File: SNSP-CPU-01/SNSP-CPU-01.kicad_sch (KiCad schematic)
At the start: 400 parts, among them J1 Jack-DC, J3 Conn_02x06_Odd_Even, J4 CONTROLLER 1, J5 CONTROLLER 2, P1 CASSETTE, P2 JST 11FE-BT-VK-N, P3 Conn_01x02_Pin, P7 JST 11FE-BT-VK-N, Q10 C2412K, Q11 C2412K, Q12 C2412K, Q13 C2412K, Q14 C2412K, Q15 C2412K, Q16 C2412K, Q17 C2412K, Q18 2SC5658, Q3 C2412K, Q4 C2412K, Q5 C2412K, Q6 C2412K, Q7 C2412K, Q8 C2412K, Q9 C2412K, SW1 KB, SW2 Old, T1 L_Coupled, U1 CPU, U10 LM324, U11 LM809, U12 L7805, U13 S-SMP, U14 S-DSP, U15 MS62256CL-10FC, U16 MS62256CL-10FC, U17 uPD6376, U18 S-CLK, U2 PPU1, U3 PPU2, U4 MS62256CL-10FC, U5 MS62256CL-10FC, U6 WRAM, U7 S-ENC, U8 CIC, X1 17.734MHz, X2 24.576MHz

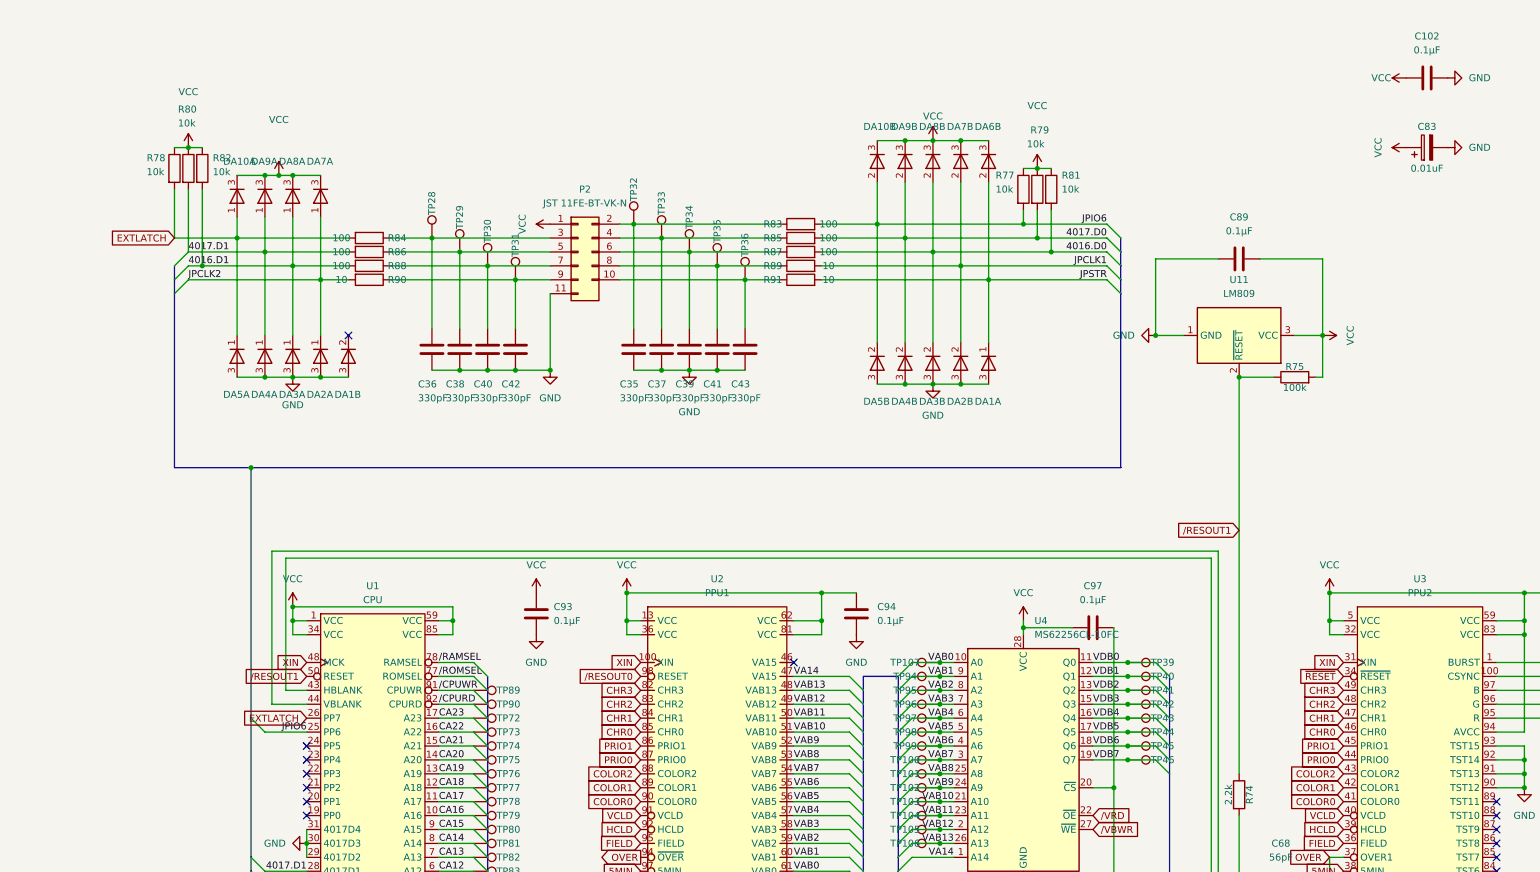
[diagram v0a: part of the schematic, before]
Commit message: front panel connector with pin names
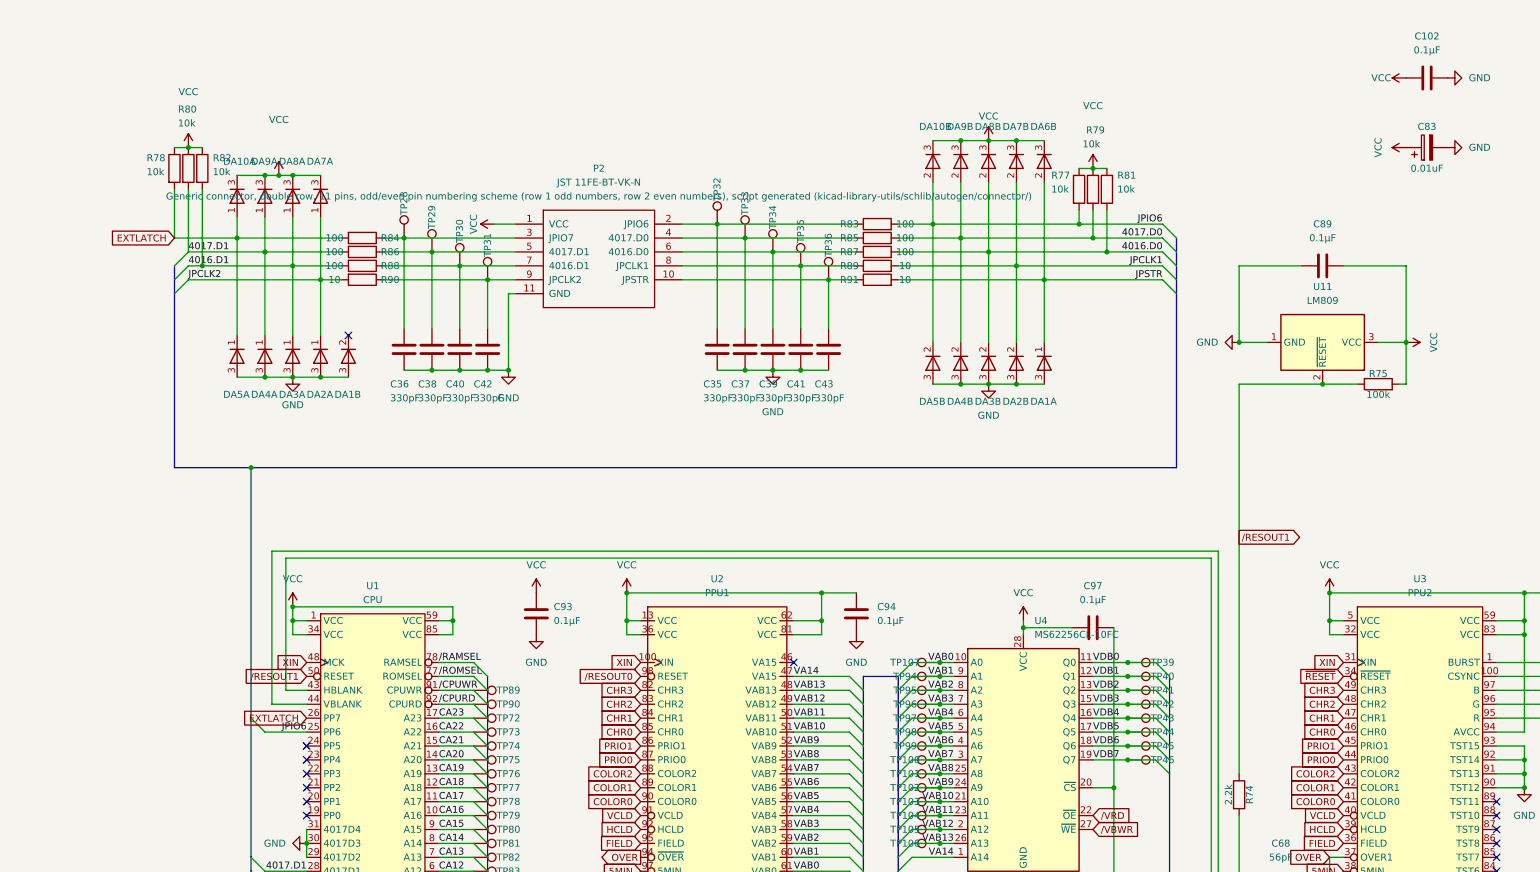
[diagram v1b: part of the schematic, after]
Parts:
- P2: symbol Connector_Generic:Conn_2Rows-11Pins -> SNES_Library:FRONT_PANEL_CONNECTOR
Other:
- moved on the sheet: C35, C36, C37, C38, C39, C40, C41, C42, C43, C89, DA10B, DA1A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
